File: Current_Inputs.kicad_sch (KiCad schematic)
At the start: 16 parts, among them J4 ANALOG VOLTAGE INPUTS, U7 D3V3XA4B10LP

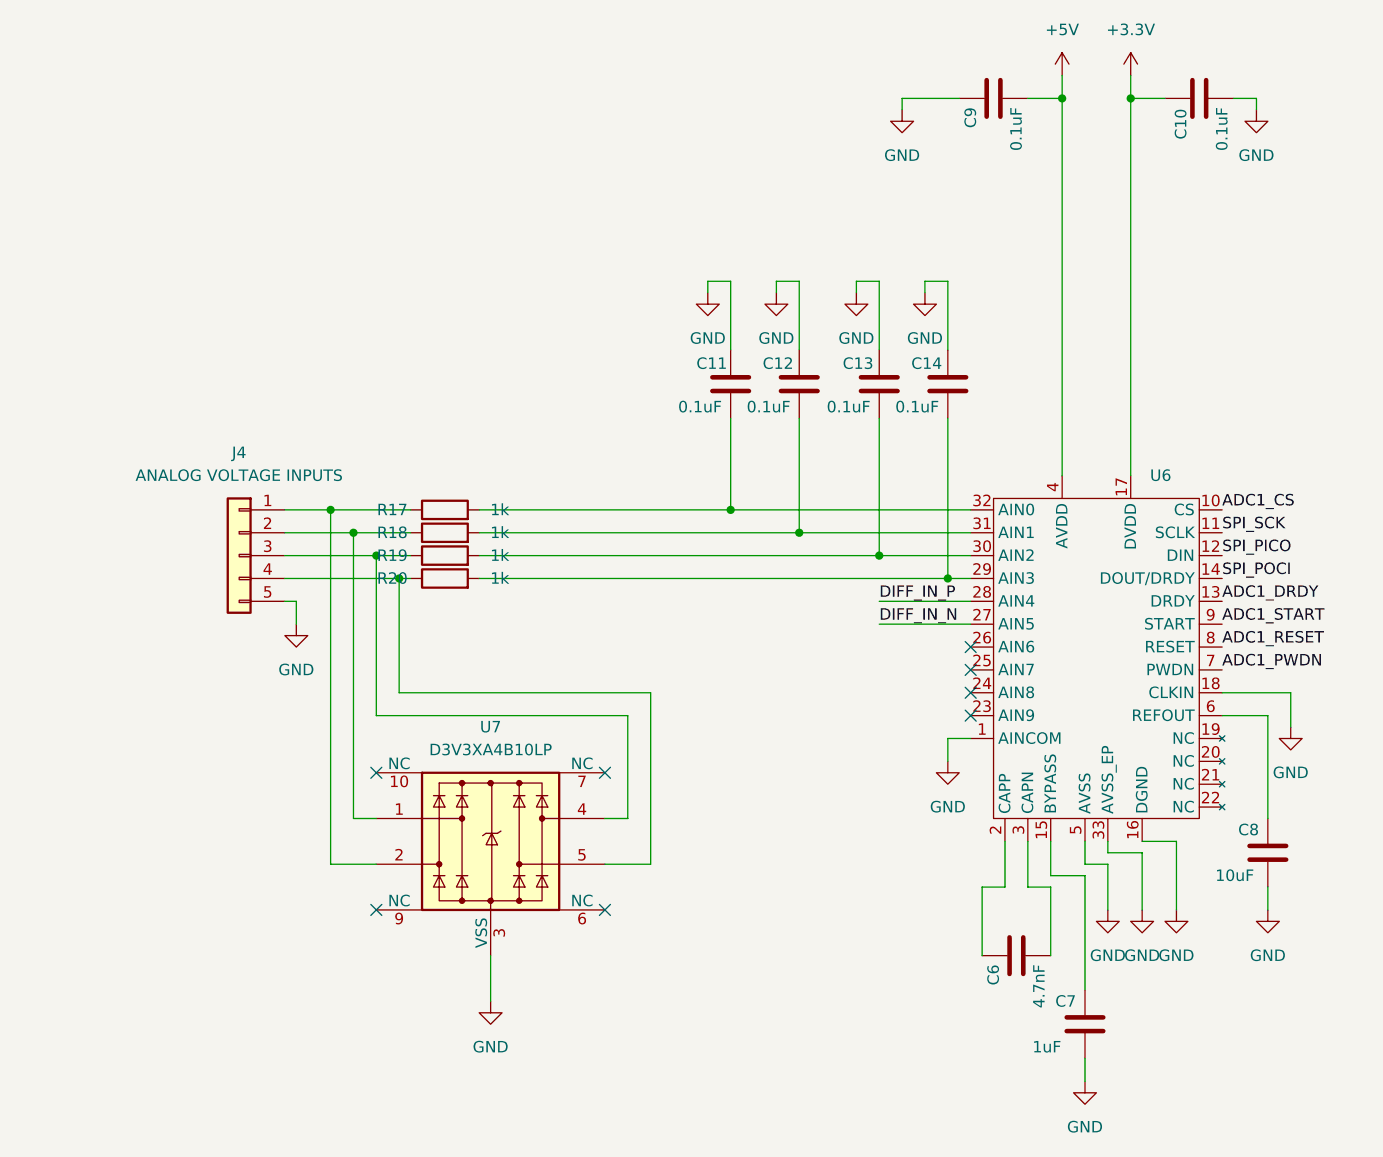
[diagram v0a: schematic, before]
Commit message: added remaining pages. BOM and refinement is all thats left
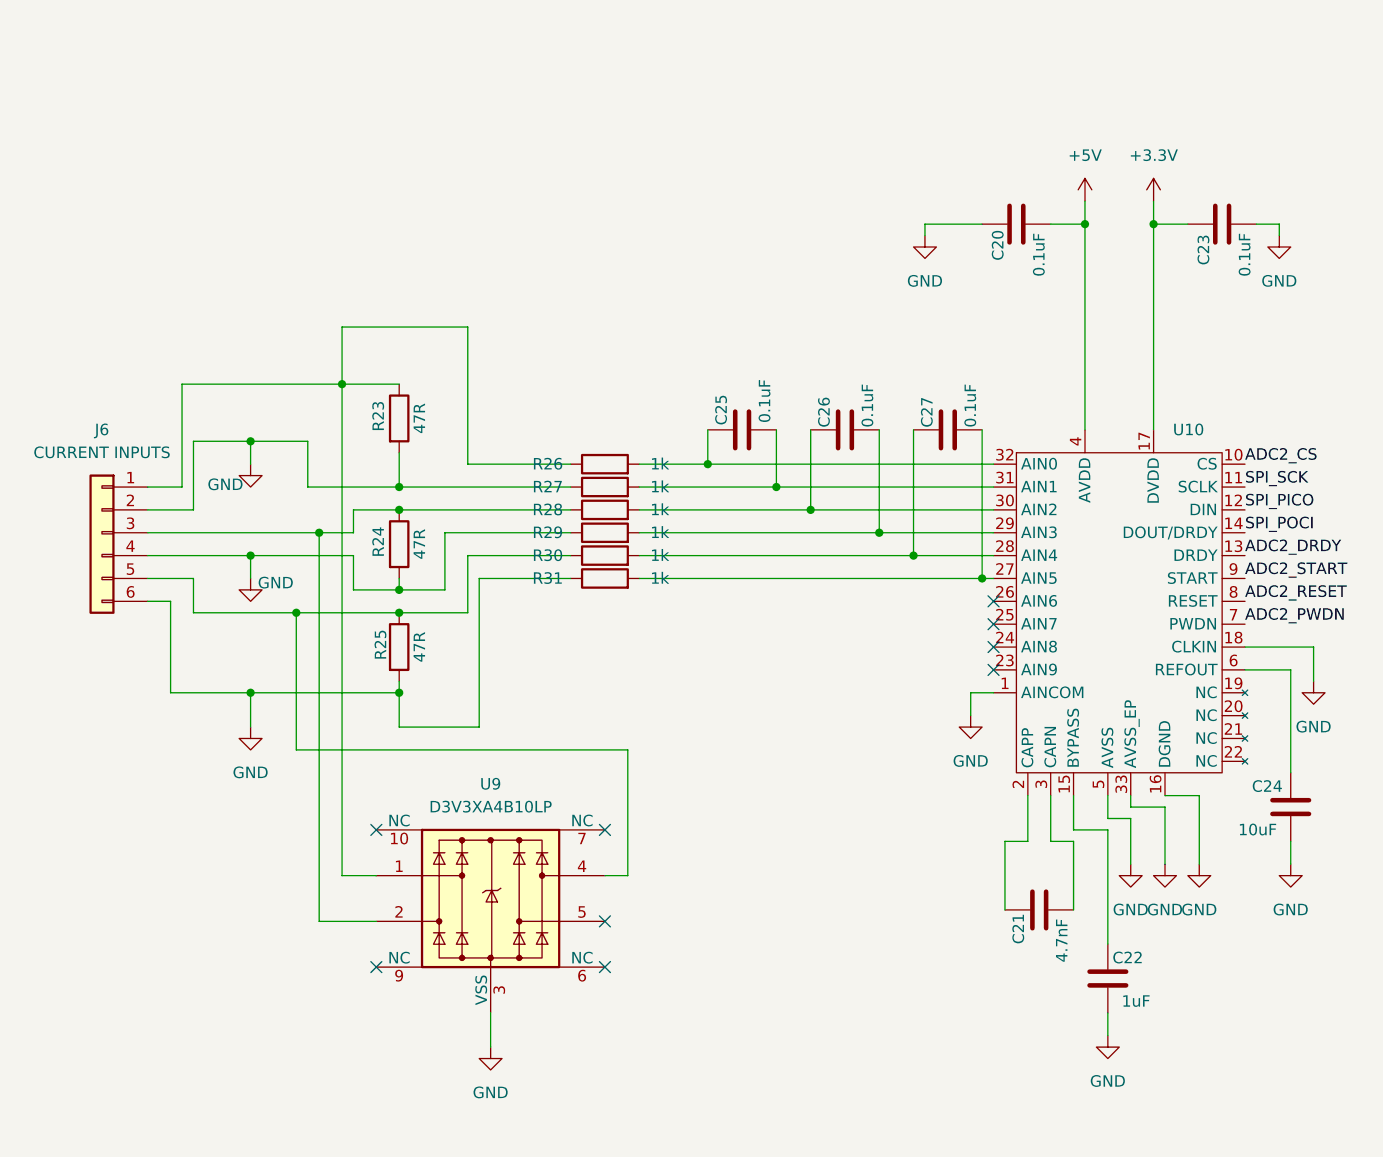
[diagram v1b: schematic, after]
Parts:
- removed C10, C11, C12, C13, C14, C9: 0.1uF, symbol Device:C
- removed C6: 4.7nF, symbol Device:C
- removed C7: 1uF, symbol Device:C
- removed C8: 10uF, symbol Device:C
- removed J4: ANALOG VOLTAGE INPUTS, symbol Connector_Generic:Conn_01x05
- removed R17, R18, R19, R20: 1k, symbol Device:R
- removed U6: (no value), Package_QFP:TQFP-64_10x10mm_P0.5mm, symbol Custom_DT1042-04SO-7:ADS1261
- removed U7: D3V3XA4B10LP, Package_DFN_QFN:Diodes_UDFN-10_1x2.5mm_P0.5mm, symbol Power_Protection:D3V3XA4B10LP
- added C20, C23, C25, C26, C27: 0.1uF, symbol Device:C
- added C21: 4.7nF, symbol Device:C
- added C22: 1uF, symbol Device:C
- added C24: 10uF, symbol Device:C
- added J6: CURRENT INPUTS, symbol Connector_Generic:Conn_01x06
- added R23, R24, R25: 47R, symbol Device:R
- added R26, R27, R28, R29, R30, R31: 1k, symbol Device:R
- added U10: (no value), Package_QFP:TQFP-64_10x10mm_P0.5mm, symbol Custom_DT1042-04SO-7:ADS1261
- added U9: D3V3XA4B10LP, Package_DFN_QFN:Diodes_UDFN-10_1x2.5mm_P0.5mm, symbol Power_Protection:D3V3XA4B10LP
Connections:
- net +3.3V: now also C23.1, U10.17 (DVDD)
- net +5V: now also C20.2, U10.4 (AVDD)
- net GND: now also C20.1, C22.2, C23.2, C24.2, J6.2 (Pin_2), J6.4 (Pin_4), J6.6 (Pin_6), R23.2, R24.2, R25.2, R27.1, R29.1, R31.1, U10.1 (AINCOM), U10.16 (DGND), U10.18 (CLKIN), U10.33 (AVSS_EP), U10.5 (AVSS), U9.3 (VSS), U9.8 (VSS)
- net SPI_PICO: now also U10.12 (DIN)
- net SPI_POCI: now also U10.14 (DOUT/DRDY)
- net SPI_SCK: now also U10.11 (SCLK)
- new net: C24.1, U10.6 (REFOUT)
- new net: C22.1, U10.15 (BYPASS)
- new net: C26.1, R28.2, U10.30 (AIN2)
- new net: C26.2, R29.2, U10.29 (AIN3)
- new net: J6.5 (Pin_5), R25.1, R30.1, U9.4
- new net: C27.1, R30.2, U10.28 (AIN4)
- new net: J6.1 (Pin_1), R23.1, R26.1, U9.1
- new net: J6.3 (Pin_3), R24.1, R28.1, U9.2
- new net: C27.2, R31.2, U10.27 (AIN5)
- new net: C21.1, U10.2 (CAPP)
- new net: C21.2, U10.3 (CAPN)
- new net: C25.2, R27.2, U10.31 (AIN1)
- new net: C25.1, R26.2, U10.32 (AIN0)
- new net ADC2_CS: U10.10 (CS)
- new net ADC2_DRDY: U10.13 (DRDY)
- new net ADC2_PWDN: U10.7 (PWDN)
- new net ADC2_RESET: U10.8 (RESET)
- new net ADC2_START: U10.9 (START)
- no-connect marks 8 -> 9
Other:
- title: Analog Voltage Inputs -> Current Inputs
